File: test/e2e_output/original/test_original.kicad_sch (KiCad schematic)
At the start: 6 parts, among them U1 R_0805_2012Metric_Pad1.20x1.4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, U2 SOT-23, U3 TO-220-3_Horizontal_TabDown, U4 TO-92_Wide, U5 R_Axial_DIN0207_L6.3mm_D2.5mm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, U6 R_Axial_DIN0207_L6.3mm_D2.5mm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

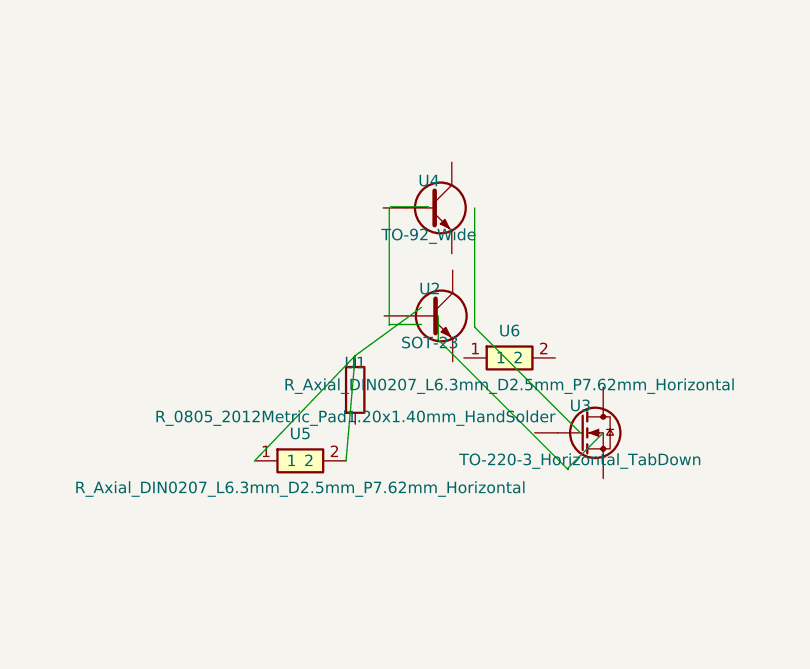
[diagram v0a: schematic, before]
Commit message: backup
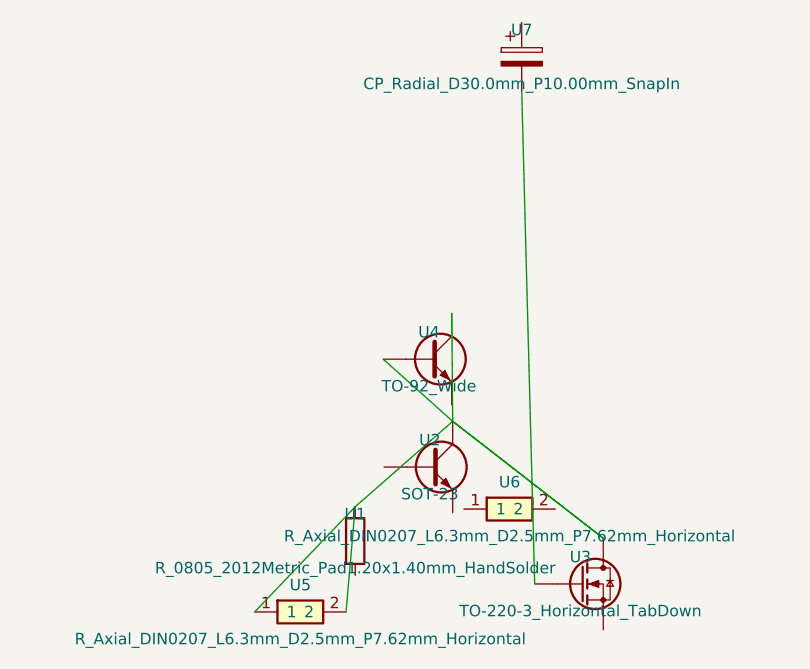
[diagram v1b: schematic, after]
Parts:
- added U7: CP_Radial_D30.0mm_P10.00mm_SnapIn, RE_passive_tht:CP_Radial_D30.0mm_P10.00mm_SnapIn, symbol RE_passive:C_Polarized
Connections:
- net at U1.1, U5.1, U5.2: now also U2.C, U3.D, U4.B, U4.C
- net at U3.G: now also U7.2
